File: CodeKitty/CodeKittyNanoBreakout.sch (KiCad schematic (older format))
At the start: 17 parts, among them P1 CONN_01X02, P2 CONN_01X02, P3 CONN_01X03, P4 CONN_01X03, P5 CONN_01X03, SW1 SW_PUSH_SMALL_H, SW2 Switch_SPDT_x2, U1 ArduinoNano

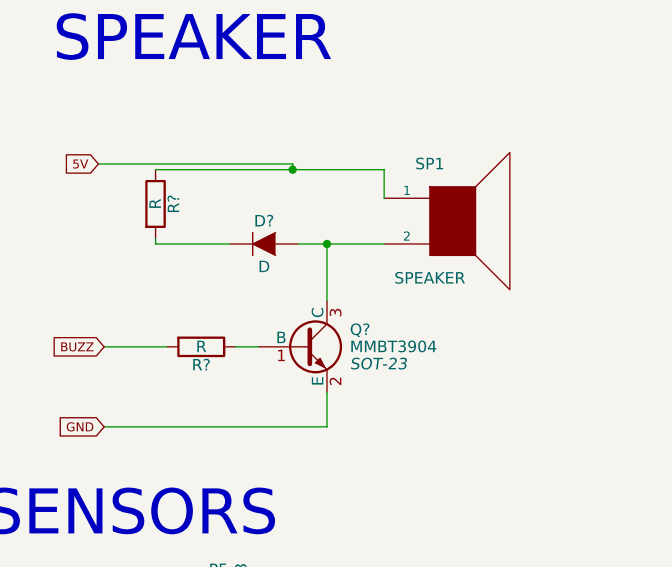
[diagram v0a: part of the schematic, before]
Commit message: ServoTester first commit
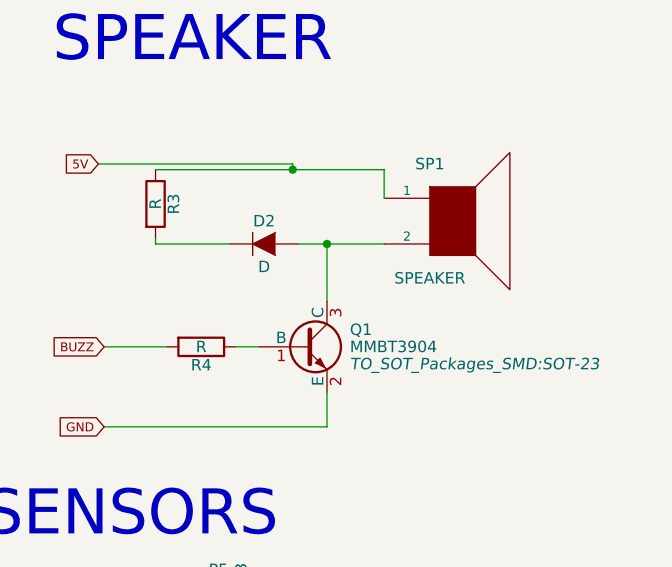
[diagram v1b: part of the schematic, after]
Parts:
- D2: renamed from D?; footprint (none) -> Diodes_SMD:D_SOD-323_HandSoldering
- Q1: renamed from Q?; footprint SOT-23 -> TO_SOT_Packages_SMD:SOT-23
- R1, R2: footprint Resistors_SMD:R_0805_HandSoldering -> Resistors_SMD:R_0603_HandSoldering
- R3, R4: renamed from R?; footprint (none) -> Resistors_SMD:R_0603_HandSoldering
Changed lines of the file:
@@
 F 0 "R2" V 6755 1650 50  0000 C CNN
 F 1 "R" V 6675 1650 50  0000 C CNN
-F 2 "Resistors_SMD:R_0805_HandSoldering" V 6605 1650 50  0001 C CNN
+F 2 "Resistors_SMD:R_0603_HandSoldering" V 6605 1650 50  0001 C CNN
 F 3 "" H 6675 1650 50  0000 C CNN
 	1    6675 1650
@@
 F 0 "R1" V 2030 3800 50  0000 C CNN
 F 1 "R" V 1950 3800 50  0000 C CNN
-F 2 "Resistors_SMD:R_0805_HandSoldering" V 1880 3800 50  0001 C CNN
+F 2 "Resistors_SMD:R_0603_HandSoldering" V 1880 3800 50  0001 C CNN
 F 3 "" H 1950 3800 50  0000 C CNN
 	1    1950 3800
@@
 5V
 $Comp
-L D D?
+L D D2
 U 1 1 5A0CCEA3
 P 9150 1650
-F 0 "D?" H 9150 1750 50  0000 C CNN
+F 0 "D2" H 9150 1750 50  0000 C CNN
 F 1 "D" H 9150 1550 50  0000 C CNN
-F 2 "" H 9150 1650 50  0000 C CNN
+F 2 "Diodes_SMD:D_SOD-323_HandSoldering" H 9150 1650 50  0001 C CNN
 F 3 "" H 9150 1650 50  0000 C CNN
 	1    9150 1650
@@
 $EndComp
 $Comp
-L R R?
+L R R3
 U 1 1 5A0CCF8E
 P 8675 1475
-F 0 "R?" V 8755 1475 50  0000 C CNN
+F 0 "R3" V 8755 1475 50  0000 C CNN
 F 1 "R" V 8675 1475 50  0000 C CNN
-F 2 "" V 8605 1475 50  0000 C CNN
+F 2 "Resistors_SMD:R_0603_HandSoldering" V 8605 1475 50  0001 C CNN
 F 3 "" H 8675 1475 50  0000 C CNN
 	1    8675 1475
@@
 $EndComp
 $Comp
-L R R?
+L R R4
 U 1 1 5A0CD00D
 P 8875 2100
-F 0 "R?" V 8955 2100 50  0000 C CNN
+F 0 "R4" V 8955 2100 50  0000 C CNN
 F 1 "R" V 8875 2100 50  0000 C CNN
-F 2 "" V 8805 2100 50  0000 C CNN
+F 2 "Resistors_SMD:R_0603_HandSoldering" V 8805 2100 50  0001 C CNN
 F 3 "" H 8875 2100 50  0000 C CNN
 	1    8875 2100
@@
 $EndComp
 $Comp
-L MMBT3904 Q?
+L MMBT3904 Q1
 U 1 1 5A0CD092
 P 9325 2100
-F 0 "Q?" H 9525 2175 50  0000 L CNN
+F 0 "Q1" H 9525 2175 50  0000 L CNN
 F 1 "MMBT3904" H 9525 2100 50  0000 L CNN
-F 2 "SOT-23" H 9525 2025 50  0000 L CIN
+F 2 "TO_SOT_Packages_SMD:SOT-23" H 9525 2025 50  0000 L CIN
 F 3 "" H 9325 2100 50  0000 L CNN
 	1    9325 2100
